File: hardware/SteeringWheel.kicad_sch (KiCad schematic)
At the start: 25 parts, among them J1 Conn_01x04, SW1 SW_Push, U4 STM32L4P5RETx, Y1 16MHz

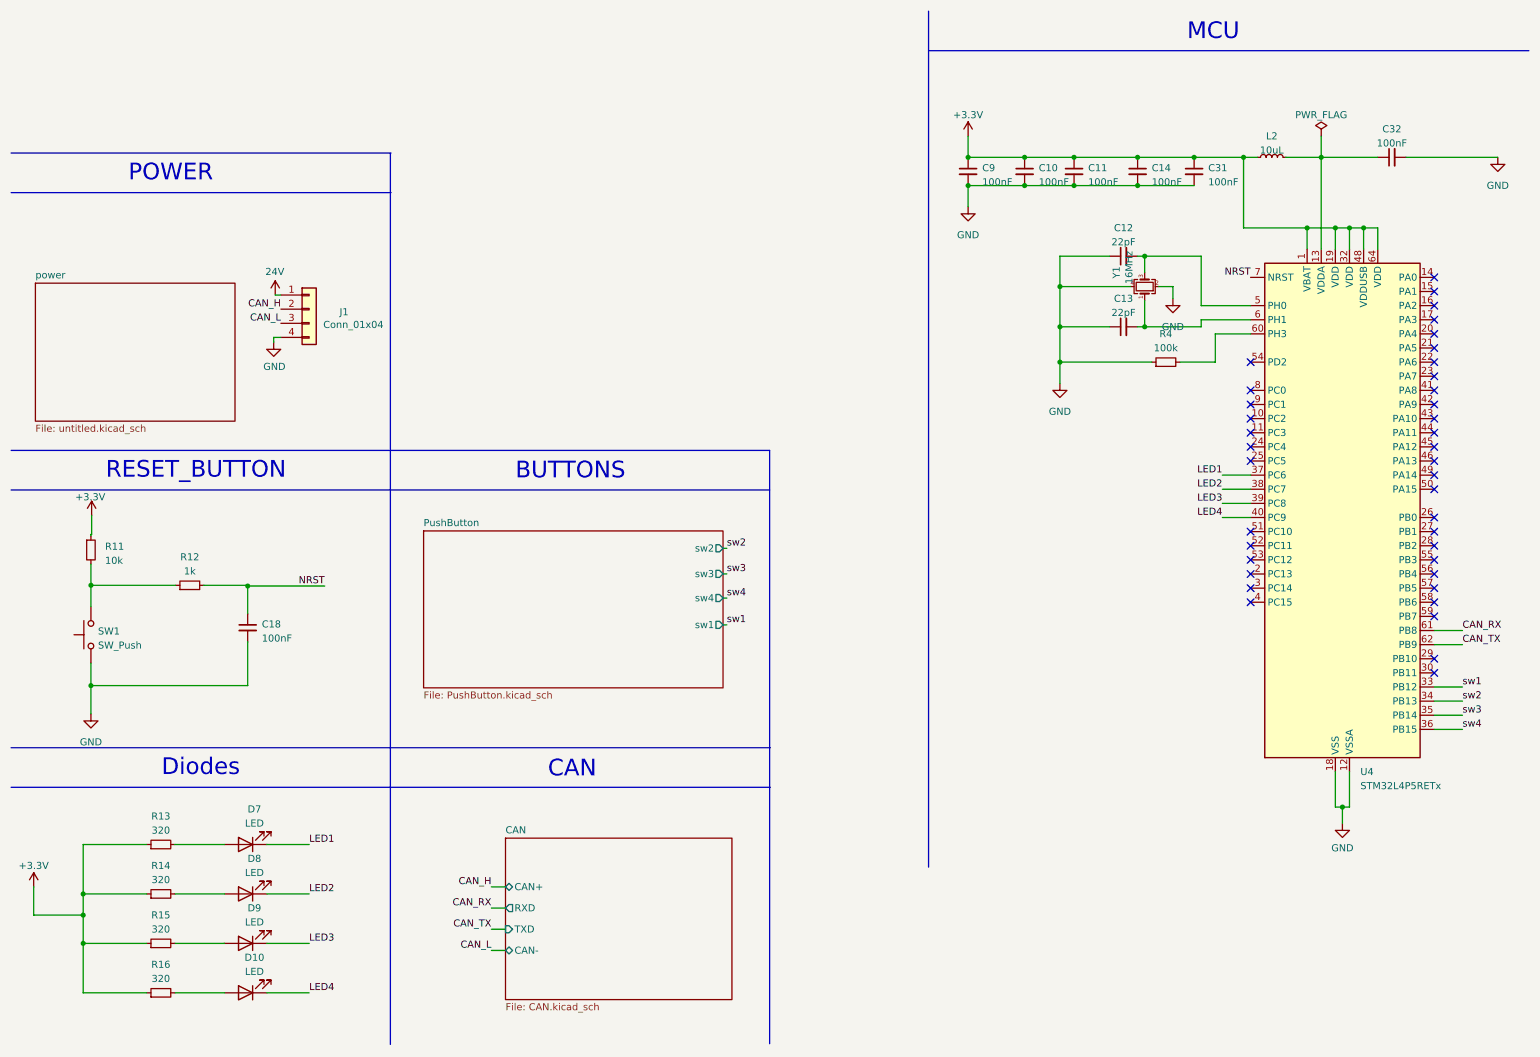
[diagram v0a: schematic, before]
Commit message: Layout done
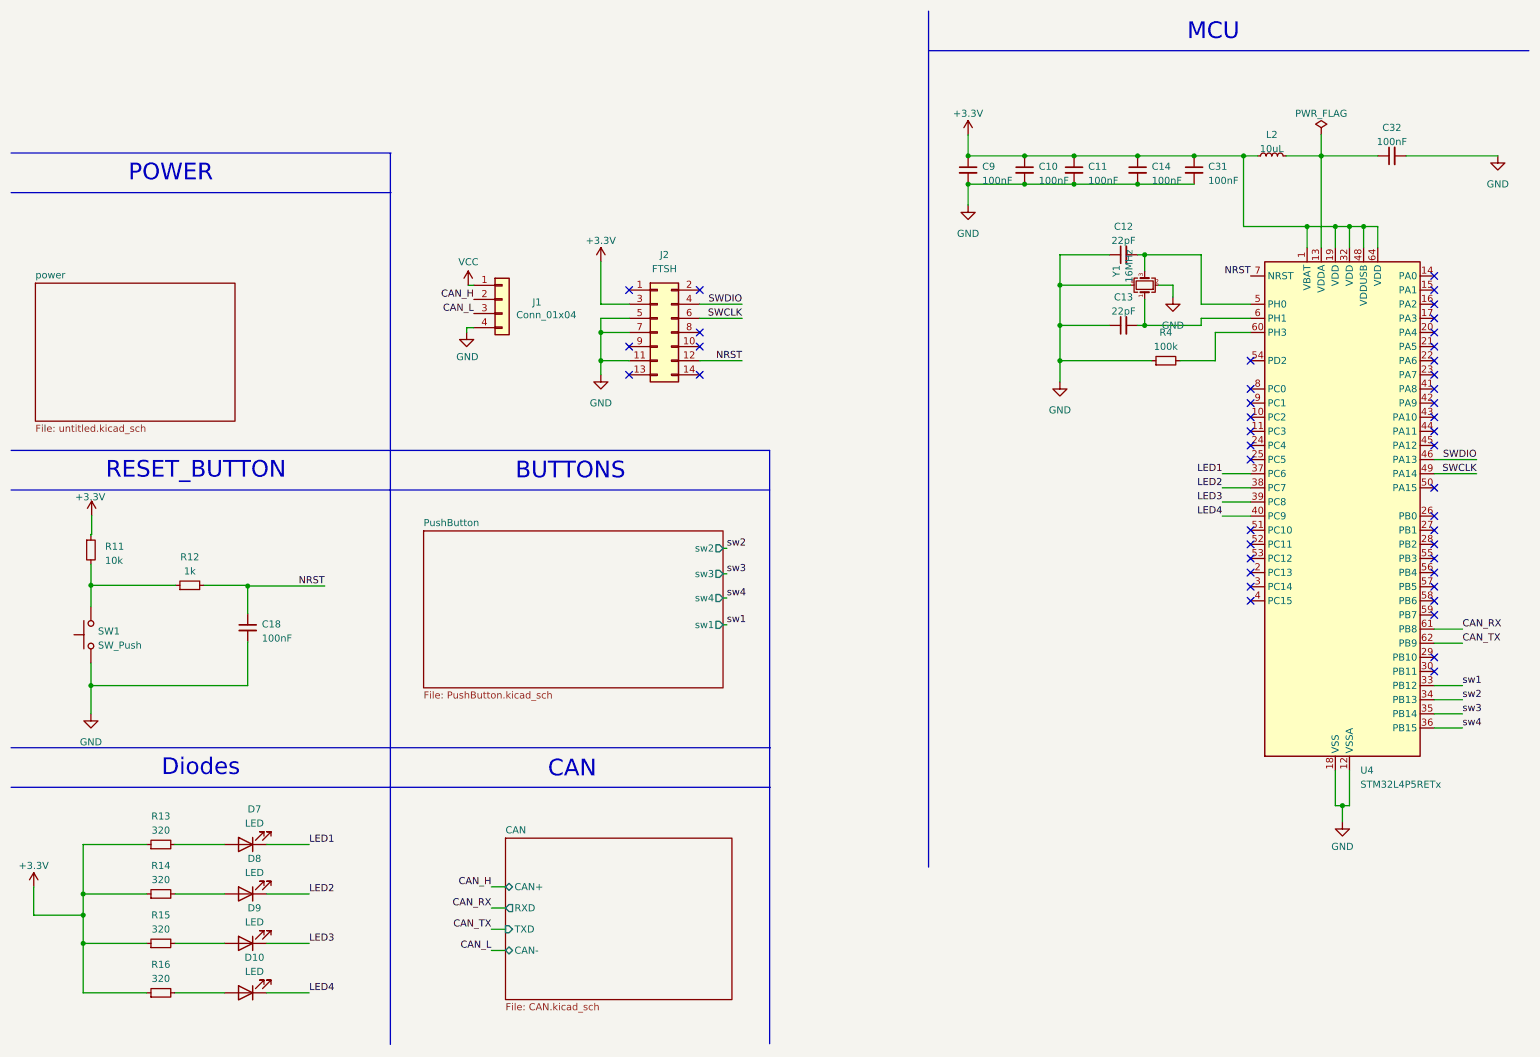
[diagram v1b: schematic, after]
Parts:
- added J2: FTSH, ftsh-107-01-l-dv-k-a:FTSH-107-XX-YYY-DV-K-A, symbol ftsh-107-01-l-dv-k-a:FTSH-107-01-L-DV-K-A
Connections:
- net +3.3V: now also J2.3 (Pin_3)
- net GND: now also J2.11 (Pin_11), J2.5 (Pin_5), J2.7 (Pin_7)
- net NRST: now also J2.12 (Pin_12)
- net SWDIO: now reaches U4.46 (PA13)
- net SWDIO: now also J2.4 (Pin_4)
- net SWCLK: now reaches U4.49 (PA14)
- net SWCLK: now also J2.6 (Pin_6)
- no-connect marks 39 -> 44
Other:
- moved on the sheet: J1

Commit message: Fix minor issues
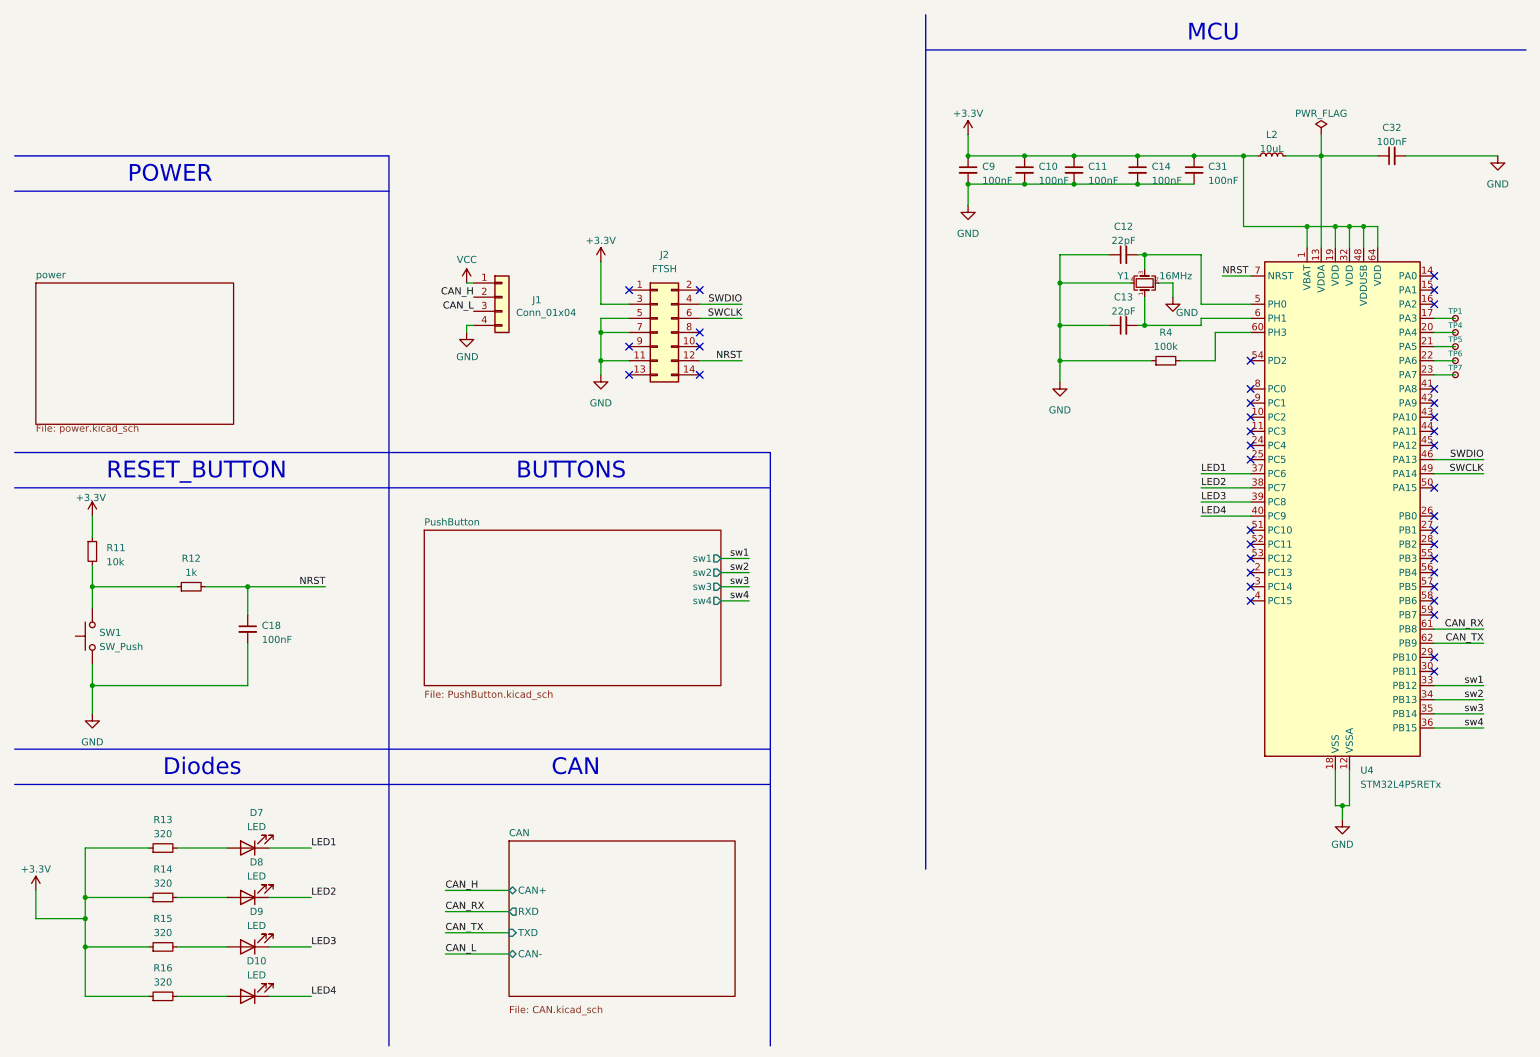
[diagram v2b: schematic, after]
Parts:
- added TP1, TP4, TP5, TP6, TP7: TestPoint_Small, TestPoint:TestPoint_Pad_D1.0mm, symbol Connector:TestPoint_Small
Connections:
- net at U4.17 (PA3): now also TP1.1
- net at U4.20 (PA4): now also TP4.1
- net at U4.21 (PA5): now also TP5.1
- net at U4.22 (PA6): now also TP6.1
- net at U4.23 (PA7): now also TP7.1
- no-connect marks 44 -> 39
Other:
- sheet power: file untitled.kicad_sch -> power.kicad_sch
- moved on the sheet: D10, D7, D8, D9, R13, R14, R15, R16
